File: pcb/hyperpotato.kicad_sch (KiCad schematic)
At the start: 43 parts, among them J1 Conn_01x02_Socket, J2 Conn_01x03_Pin, Q1 AO3401A, SW1 SW_Push_45deg, SW10 SW_Push_45deg, SW11 SW_Push_45deg, SW12 SW_Push_45deg, SW13 SW_Push_45deg, SW14 SW_SPDT, SW15 SW_Push, SW2 SW_Push_45deg, SW3 SW_Push_45deg, SW4 SW_Push_45deg, SW5 SW_Push_45deg, SW6 SW_Push_45deg, SW7 SW_Push_45deg, SW8 SW_Push_45deg, SW9 SW_Push_45deg, U1 Seeeduino Xiao nRF52840, U2 SK8707-01-SENSOR, U3 SK8707-01, U4 DRV2605LDGS, U5 74HC595

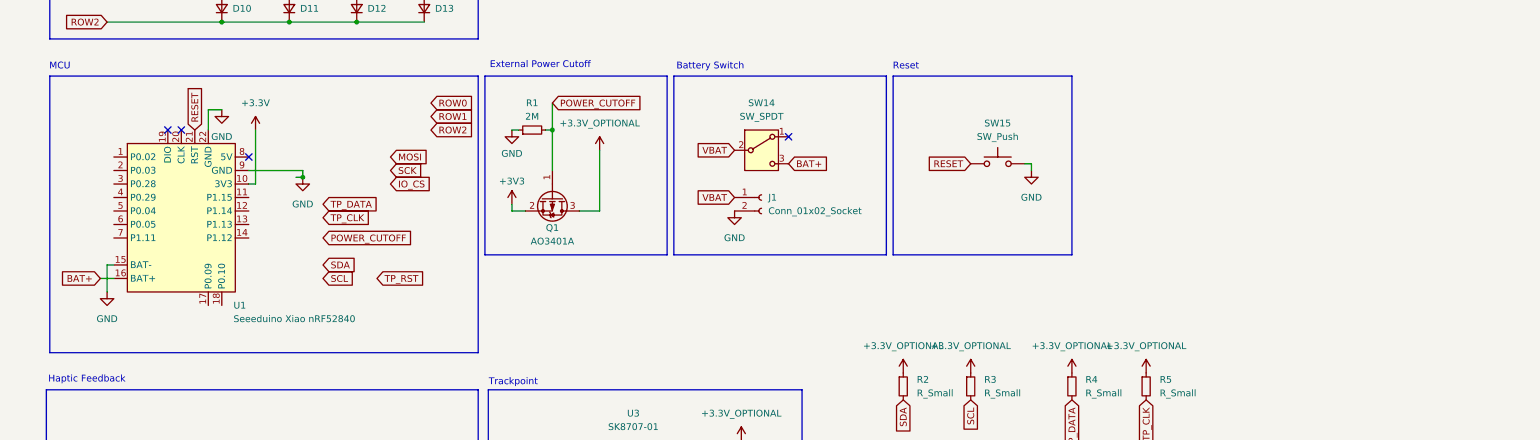
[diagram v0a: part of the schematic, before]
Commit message: Finish wiring
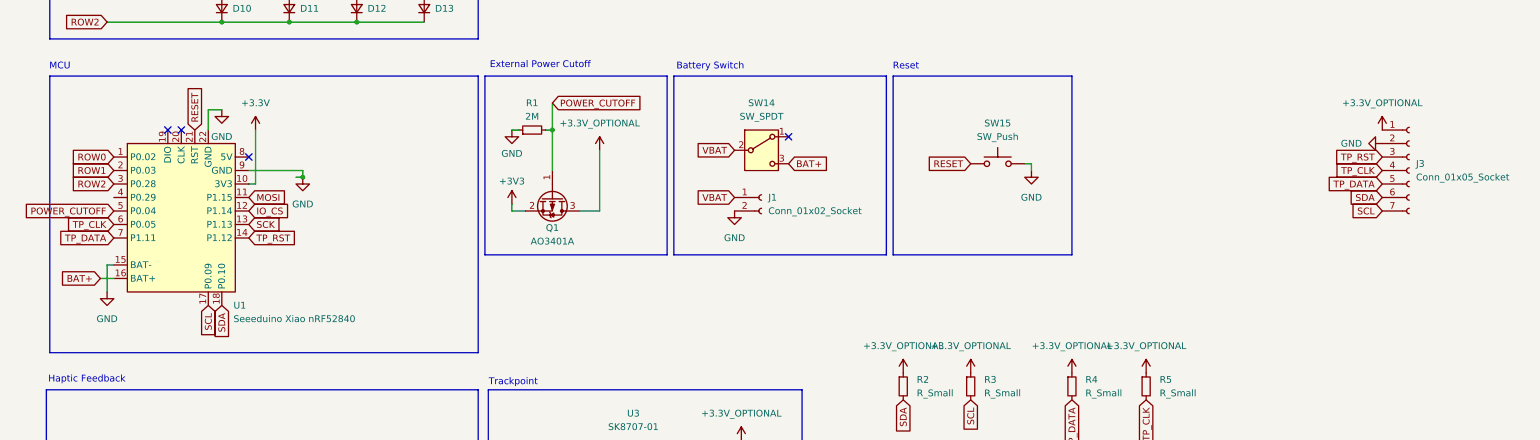
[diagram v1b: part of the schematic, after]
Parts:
- added J3: Conn_01x05_Socket, Connector_PinHeader_2.54mm:PinHeader_1x07_P2.54mm_Vertical, symbol Connector:Conn_01x07_Socket
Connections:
- net +3.3V_OPTIONAL: now also J3.1 (Pin_1)
- net GND: now also J3.2 (Pin_2)
- net IO_CS: now also U1.12 (P1.14)
- net MOSI: now also U1.11 (P1.15)
- net POWER_CUTOFF: now also U1.5 (P0.04)
- net ROW0: now also U1.1 (P0.02)
- net ROW1: now also U1.2 (P0.03)
- net ROW2: now also U1.3 (P0.28)
- net SCK: now also U1.13 (P1.13)
- net SCL: now also U1.17 (P0.09), J3.7 (Pin_7)
- net SDA: now also U1.18 (P0.10), J3.6 (Pin_6)
- net TP_CLK: now also U1.6 (P0.05), J3.4 (Pin_4)
- net TP_DATA: now also U1.7 (P1.11), J3.5 (Pin_5)
- net TP_RST: now also U1.14 (P1.12), J3.3 (Pin_3)
